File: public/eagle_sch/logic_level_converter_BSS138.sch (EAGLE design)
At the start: 3 parts, among them Q1 BSS138

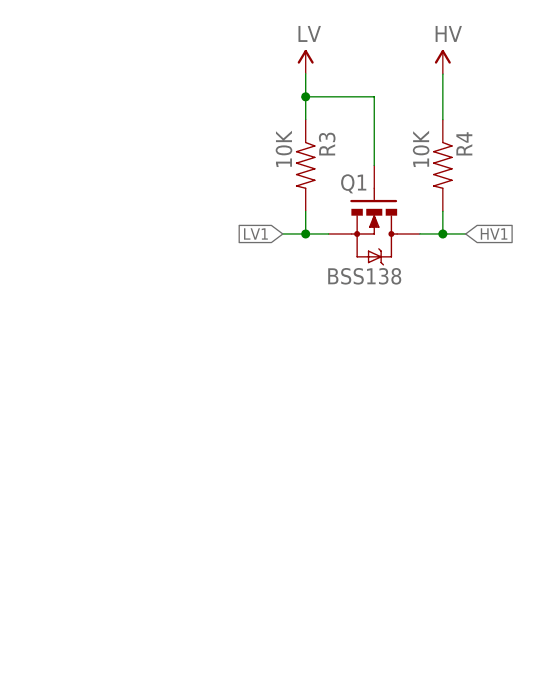
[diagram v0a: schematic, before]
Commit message: download sch
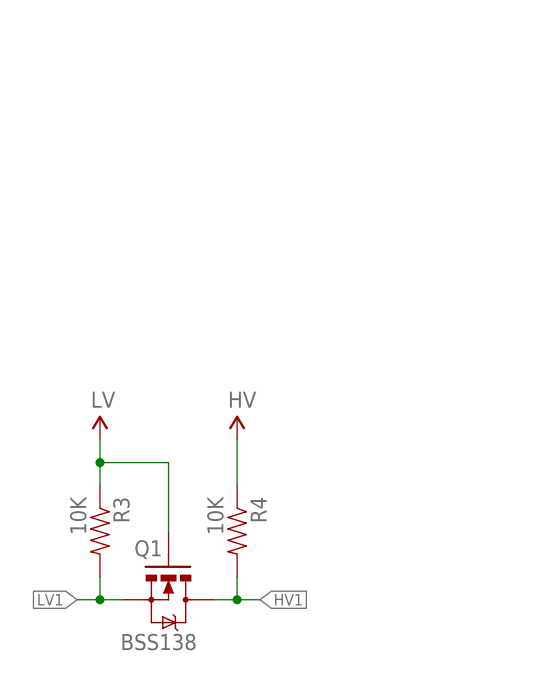
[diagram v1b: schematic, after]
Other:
- moved on the sheet: Q1, R3, R4
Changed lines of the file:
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@@
 <?xml version="1.0" encoding="utf-8"?>
 <!DOCTYPE eagle SYSTEM "eagle.dtd">
-<eagle version="6.1">
+<eagle version="6.4">
 <drawing>
 <settings>
@@
 <part name="P+1" library="SparkFun" deviceset="VCC" device="" value="LV"/>
 <part name="P+4" library="SparkFun" deviceset="VCC" device="" value="HV"/>
-<part name="FRAME1" library="SparkFun-Aesthetics" deviceset="FRAME-A4L" device=""/>
 </parts>
 <sheets>
@@
 </plain>
 <instances>
-<instance part="Q1" gate="G$1" x="43.18" y="50.8" smashed="yes" rot="R270">
-<attribute name="NAME" x="39.37" y="55.626" size="1.778" layer="95"/>
-<attribute name="VALUE" x="37.846" y="45.212" size="1.778" layer="96"/>
+<instance part="Q1" gate="G$1" x="20.32" y="10.16" smashed="yes" rot="R270">
+<attribute name="NAME" x="16.51" y="14.986" size="1.778" layer="95"/>
+<attribute name="VALUE" x="14.986" y="4.572" size="1.778" layer="96"/>
 </instance>
-<instance part="R3" gate="G$1" x="35.56" y="58.42" rot="R270"/>
-<instance part="R4" gate="G$1" x="50.8" y="58.42" rot="R270"/>
-<instance part="P+1" gate="1" x="35.56" y="68.58"/>
-<instance part="P+4" gate="1" x="50.8" y="68.58"/>
-<instance part="FRAME1" gate="G$1" x="-91.44" y="-30.48"/>
+<instance part="R3" gate="G$1" x="12.7" y="17.78" rot="R270"/>
+<instance part="R4" gate="G$1" x="27.94" y="17.78" rot="R270"/>
+<instance part="P+1" gate="1" x="12.7" y="27.94"/>
+<instance part="P+4" gate="1" x="27.94" y="27.94"/>
 </instances>
 <busses>
@@
 <net name="LV" class="0">
 <segment>
-<wire x1="35.56" y1="63.5" x2="35.56" y2="66.04" width="0.1524" layer="91"/>
-<wire x1="35.56" y1="66.04" x2="35.56" y2="68.58" width="0.1524" layer="91"/>
-<wire x1="43.18" y1="58.42" x2="43.18" y2="66.04" width="0.1524" layer="91"/>
-<wire x1="43.18" y1="66.04" x2="35.56" y2="66.04" width="0.1524" layer="91"/>
-<junction x="35.56" y="66.04"/>
+<wire x1="12.7" y1="22.86" x2="12.7" y2="25.4" width="0.1524" layer="91"/>
+<wire x1="12.7" y1="25.4" x2="12.7" y2="27.94" width="0.1524" layer="91"/>
+<wire x1="20.32" y1="17.78" x2="20.32" y2="25.4" width="0.1524" layer="91"/>
+<wire x1="20.32" y1="25.4" x2="12.7" y2="25.4" width="0.1524" layer="91"/>
+<junction x="12.7" y="25.4"/>
 <pinref part="R3" gate="G$1" pin="1"/>
 <pinref part="P+1" gate="1" pin="VCC"/>
@@
 <net name="HV1" class="0">
 <segment>
-<wire x1="48.26" y1="50.8" x2="50.8" y2="50.8" width="0.1524" layer="91"/>
-<wire x1="50.8" y1="50.8" x2="53.34" y2="50.8" width="0.1524" layer="91"/>
-<wire x1="50.8" y1="53.34" x2="50.8" y2="50.8" width="0.1524" layer="91"/>
-<junction x="50.8" y="50.8"/>
+<wire x1="25.4" y1="10.16" x2="27.94" y2="10.16" width="0.1524" layer="91"/>
+<wire x1="27.94" y1="10.16" x2="30.48" y2="10.16" width="0.1524" layer="91"/>
+<wire x1="27.94" y1="12.7" x2="27.94" y2="10.16" width="0.1524" layer="91"/>
+<junction x="27.94" y="10.16"/>
 <pinref part="Q1" gate="G$1" pin="D"/>
 <pinref part="R4" gate="G$1" pin="2"/>
-<label x="53.34" y="50.8" size="1.27" layer="95" xref="yes"/>
+<label x="30.48" y="10.16" size="1.27" layer="95" xref="yes"/>
 </segment>
 </net>
 <net name="HV" class="0">
 <segment>
-<wire x1="50.8" y1="63.5" x2="50.8" y2="68.58" width="0.1524" layer="91"/>
+<wire x1="27.94" y1="22.86" x2="27.94" y2="27.94" width="0.1524" layer="91"/>
 <pinref part="R4" gate="G$1" pin="1"/>
 <pinref part="P+4" gate="1" pin="VCC"/>
@@
 <net name="LV1" class="0">
 <segment>
-<wire x1="38.1" y1="50.8" x2="35.56" y2="50.8" width="0.1524" layer="91"/>
-<wire x1="35.56" y1="50.8" x2="33.02" y2="50.8" width="0.1524" layer="91"/>
-<wire x1="35.56" y1="53.34" x2="35.56" y2="50.8" width="0.1524" layer="91"/>
-<junction x="35.56" y="50.8"/>
+<wire x1="15.24" y1="10.16" x2="12.7" y2="10.16" width="0.1524" layer="91"/>
+<wire x1="12.7" y1="10.16" x2="10.16" y2="10.16" width="0.1524" layer="91"/>
+<wire x1="12.7" y1="12.7" x2="12.7" y2="10.16" width="0.1524" layer="91"/>
+<junction x="12.7" y="10.16"/>
 <pinref part="Q1" gate="G$1" pin="S"/>
 <pinref part="R3" gate="G$1" pin="2"/>
-<label x="33.02" y="50.8" size="1.27" layer="95" rot="R180" xref="yes"/>
+<label x="10.16" y="10.16" size="1.27" layer="95" rot="R180" xref="yes"/>
 </segment>
 </net>
